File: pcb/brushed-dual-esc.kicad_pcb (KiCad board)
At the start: 2 copper layers, 29.5 x 25 mm, 26 parts, among them J1 XT30PW-M, J2 Conn_02x03_Odd_Even, J3 TC2030-NL, J6 XT30PW-F, J7 XT30PW-F, U2 AZ1117-5.0, U3 STM32C011F4Ux, U4 DRV8231ADSGR, U5 TLV77133PDBVR, U6 DRV8231ADSGR

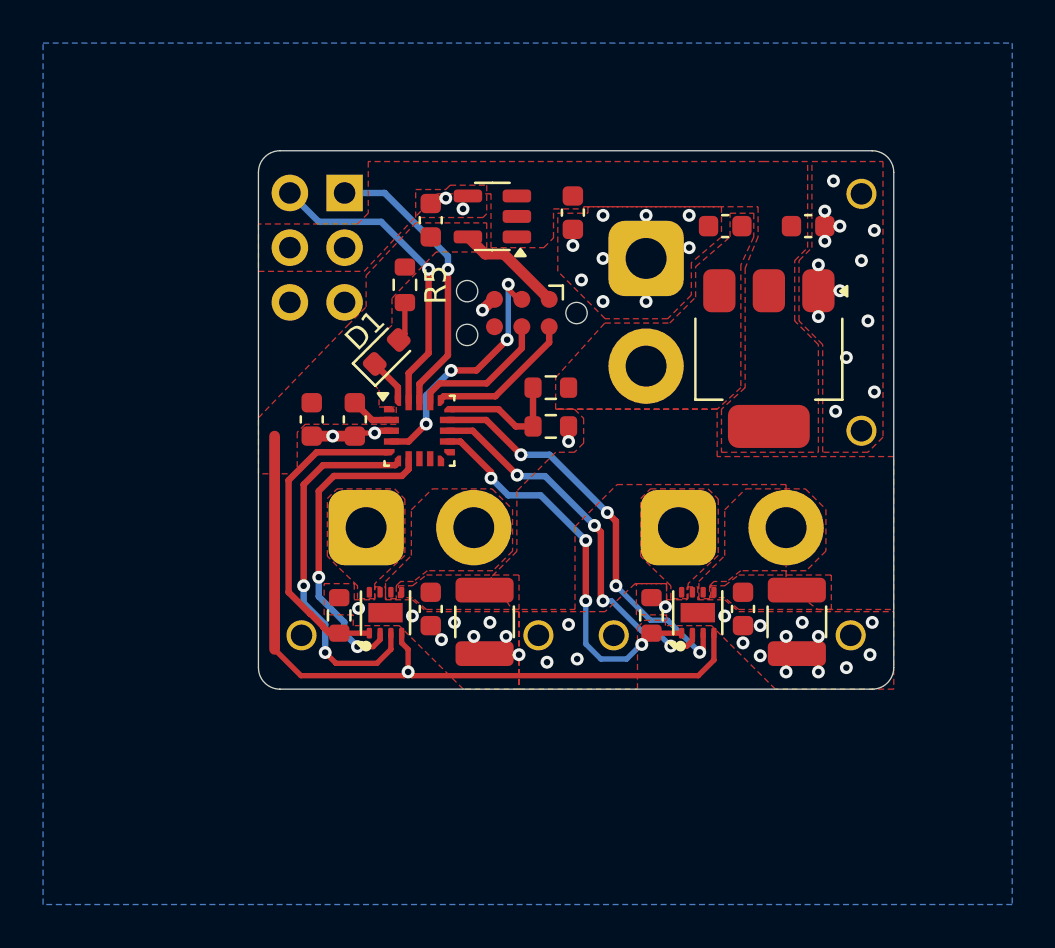
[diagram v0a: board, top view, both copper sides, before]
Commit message: Fix capacitor siutation
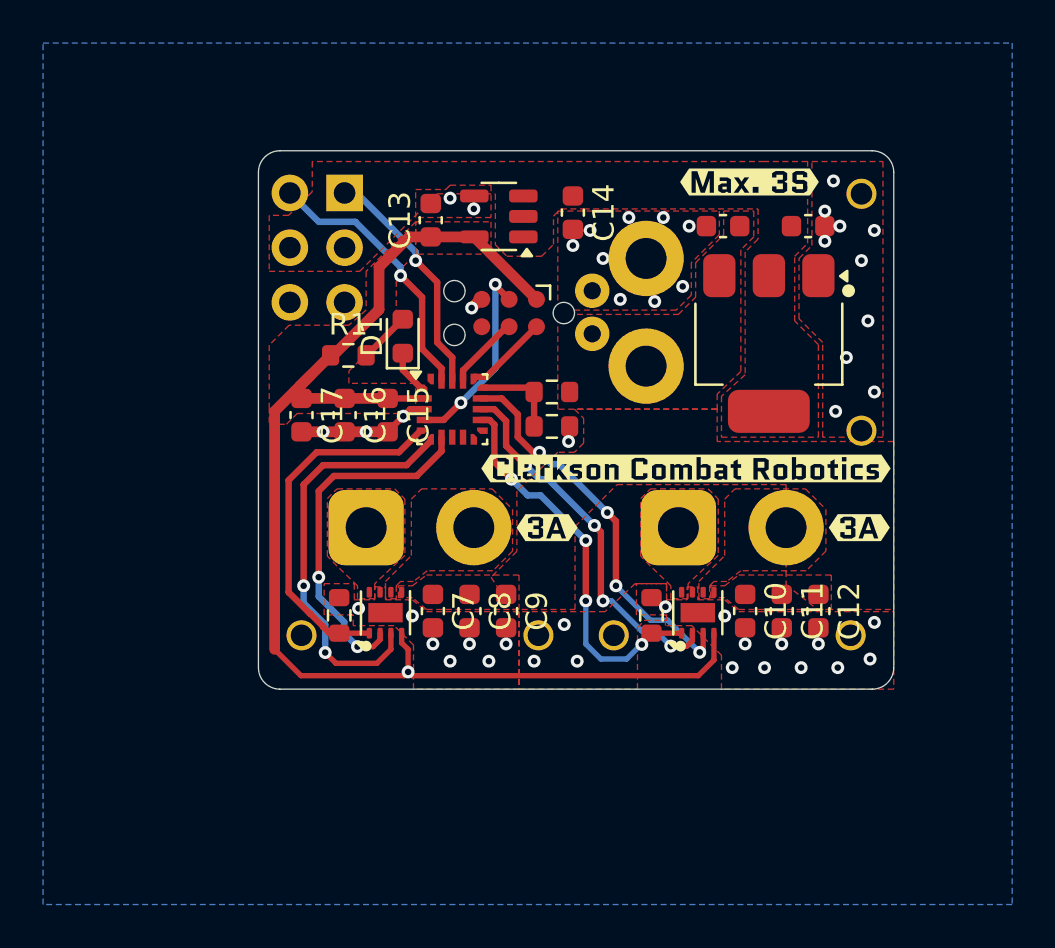
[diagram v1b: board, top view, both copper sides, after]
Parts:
- removed the C1 at (128.0, 96.3)
- removed the C3 at (142.5, 96.3)
- removed C4: 47u, Capacitor_SMD:C_1210_3225Metric
- added C10: UMK107BJ105KA-T, Capacitor_SMD:C_0603_1608Metric, F.Cu at (142.6, 96.4)
- added C11: UMK107BJ105KA-T, Capacitor_SMD:C_0603_1608Metric, F.Cu at (144.3, 96.4)
- added C12: UMK107BJ105KA-T, Capacitor_SMD:C_0603_1608Metric, F.Cu at (146.0, 96.4)
- added C13: UMK107BJ105KA-T, Capacitor_SMD:C_0603_1608Metric, F.Cu at (128.0, 78.2)
- added C16: UMK107BJ105KA-T, Capacitor_SMD:C_0603_1608Metric, F.Cu at (124.0, 87.3)
- added C17: UMK107BJ105KA-T, Capacitor_SMD:C_0603_1608Metric, F.Cu at (122.0, 87.3)
- added C7: UMK107BJ105KA-T, Capacitor_SMD:C_0603_1608Metric, F.Cu at (128.1, 96.4)
- added G***: LOGO, LOGO, B.Cu at (134.6, 89.3)
- added kibuzzard-68AE1D03: G***, kibuzzard-68AE1D03, B.Cu at (127.7, 82.0)
- added kibuzzard-68AE1D1E: G***, kibuzzard-68AE1D1E, B.Cu at (127.7, 79.5)
- added kibuzzard-68AE1D34: G***, kibuzzard-68AE1D34, B.Cu at (121.5, 85.8)
- added kibuzzard-68AE1D4C: G***, kibuzzard-68AE1D4C, B.Cu at (124.0, 85.8)
- added kibuzzard-68AE1DA9: G***, kibuzzard-68AE1DA9, B.Cu at (127.7, 77.0)
- added kibuzzard-68AE251B: G***, kibuzzard-68AE251B, F.Cu at (139.8, 89.8)
- added kibuzzard-68AE2565: G***, kibuzzard-68AE2565, F.Cu at (142.8, 76.5)
- added kibuzzard-68AE2599: G***, kibuzzard-68AE2599, F.Cu at (147.9, 92.5)
- added kibuzzard-68AE2599: G***, kibuzzard-68AE2599, F.Cu at (133.4, 92.5)
- C1: renamed from C13; value 22u -> 22u 16V
- C14, C15: value 1u -> UMK107BJ105KA-T
- C2: value 47u -> ESS107M016AC2KA; footprint Capacitor_SMD:C_1210_3225Metric -> Capacitor_THT:CP_Radial_D5.0mm_P2.00mm; moved to B.Cu
- C3: renamed from C12; value 22u -> 22u 16V
- C8: value 100n -> UMK107BJ105KA-T
- C9: value 4.7u -> UMK107BJ105KA-T
- moved C2 14.3 mm to (135.5, 83.5), turned to 90 degrees
- moved C9 12.7 mm to (131.5, 96.4)
- moved C8 10.4 mm to (129.8, 96.4)
- moved C15 9.27 mm to (126.0, 87.3), turned to -90 degrees
- moved R1 4.20 mm to (124.2, 84.5), turned to 0 degrees
- moved U3 1.82 mm to (129.0, 87.0)
- moved D1 1.04 mm to (126.7, 83.6), turned to 90 degrees
- moved U1 0.70 mm to (143.7, 84.0)
- moved J2 0.59 mm to (131.6, 82.5)
- moved U2 0.30 mm to (131.2, 78.0)
- moved R2 0.21 mm to (133.6, 86.2)
- moved C1 0.10 mm to (141.6, 78.5)
- moved R3 0.05 mm to (133.6, 87.8)
- renumbered J3 to J2, J2 to J3, J6 to J4, J7 to J5, R5 to R1, R1 to R2, R2 to R3, R3 to R4, R4 to R5, U2 to U1, U5 to U2, U6 to U5
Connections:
- C8 pad 1: +3V3 -> +BATT
- C9 pad 1: +3V3 -> +BATT
- U3 pad 1: unconnected-(U3-PC15-Pad1) -> /LED
- U3 pad 20: /LED -> unconnected-(U3-PC14-Pad20)
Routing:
- net +3V3: track 41.9 -> 60.6 mm
- net /SWCLK: track 6.57 -> 3.48 mm
- net /SWDIO: track 6.84 -> 3.89 mm
- net /~{RESET}: track 11.9 -> 9.16 mm, vias 4 -> 2
- net /RX_CH2: track 13.4 -> 11.1 mm
- net GND: track 5.34 -> 7.49 mm, vias 52 -> 47
- net /DRV1_IN2: track 14.5 -> 16.6 mm
- net /DRV1_ISENSE: track 14.9 -> 16.8 mm
- net /DRV1_IN1: track 17.3 -> 19.2 mm
- net /BATT_SENSE: track 5.93 -> 4.01 mm
- net /RX_CH1: track 14.5 -> 12.7 mm
- net Net-(D1-A): track 1.85 -> 2.39 mm
